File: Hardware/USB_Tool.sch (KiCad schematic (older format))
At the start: 39 parts, among them J1 USB_B_Micro, J2 CONN_ICSP, J3 Extender_I2C_1, J4 Extender_I2C_2, J5 Extender_I2C_3, P1 2V, P2 2V, P3 2V, P4 2V, SW1 SW_2TO1, U1 MRF89XAM8A, U2 NCP114, U3 MCP2210, U4 PIC18F45K40_44, X1 EXTENDER_SPI_1, X2 EXTENDER_IO_1, X3 EXTENDER_IO_2, X4 EXTENDER_IO_3, Y1 DSC6003JI2A

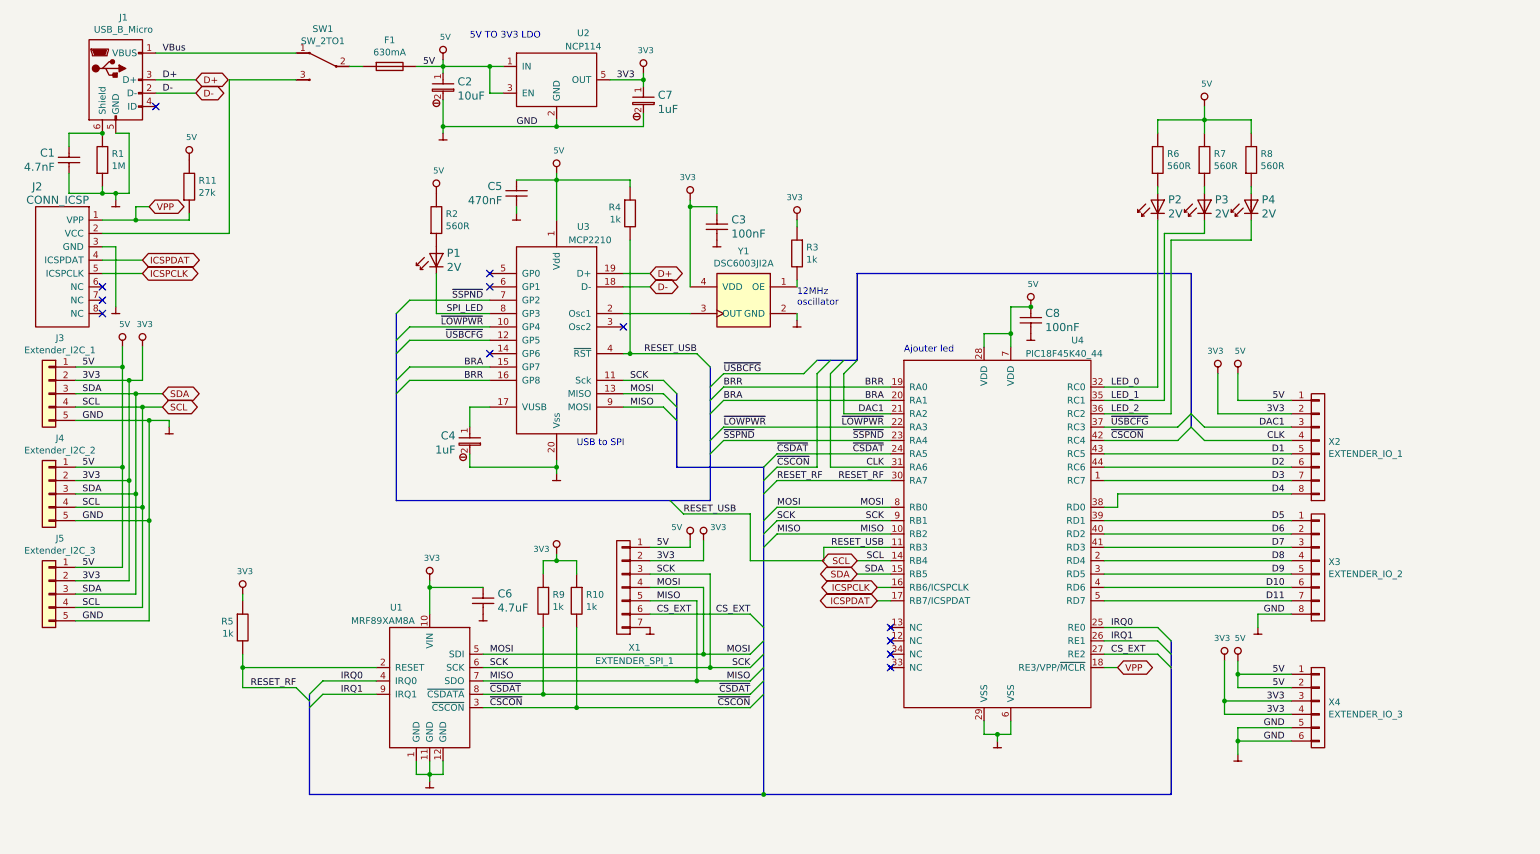
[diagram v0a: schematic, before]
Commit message: tbd
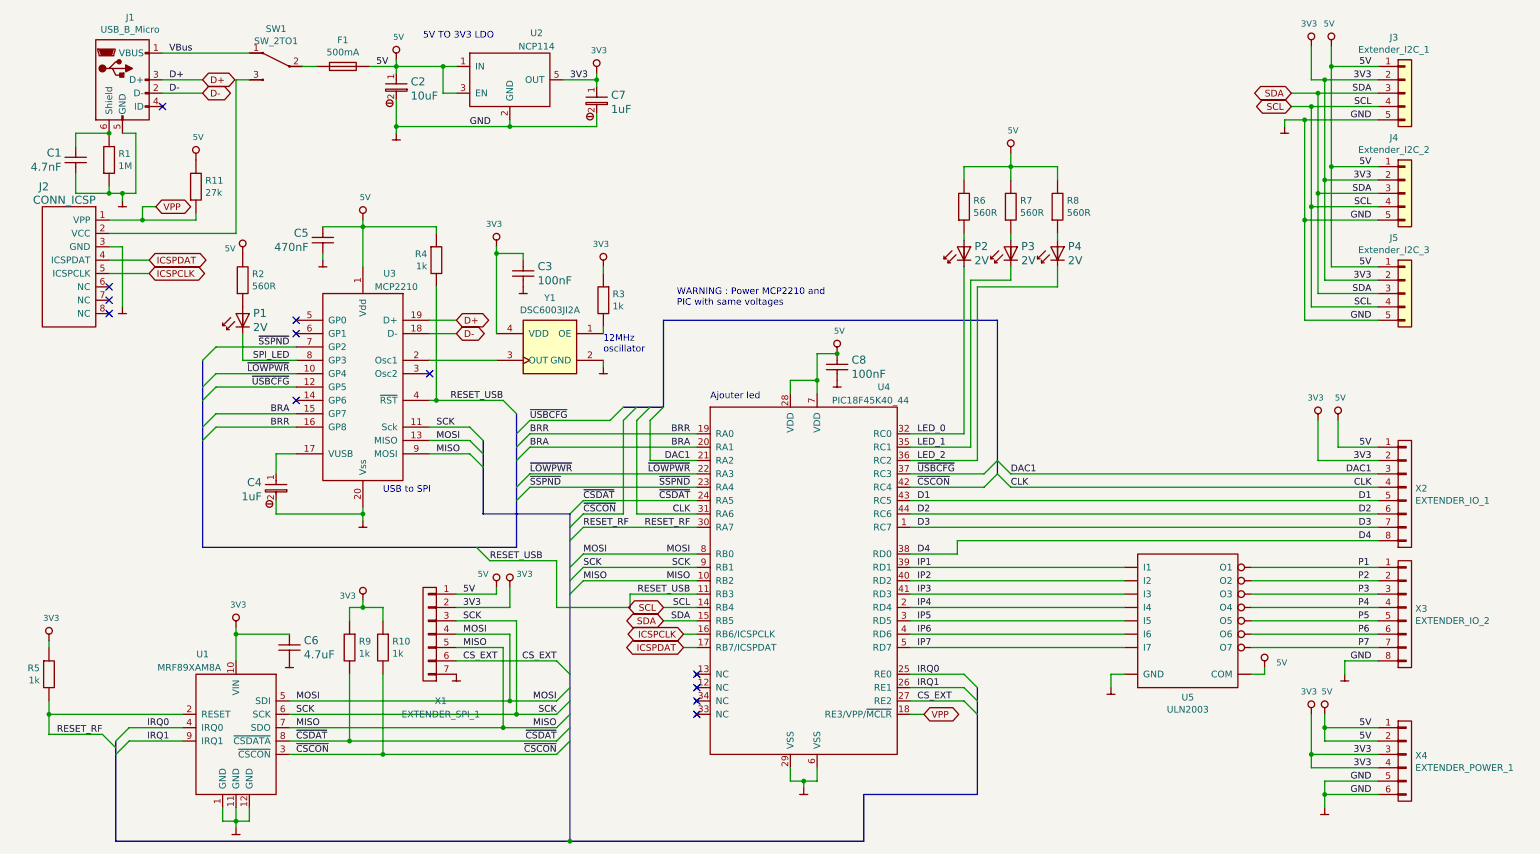
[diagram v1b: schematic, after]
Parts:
- added U5: ULN2003, symbol 0EsseivaN_Lib:ULN200x
- F1: value 630mA -> 500mA
- X4: value EXTENDER_IO_3 -> EXTENDER_POWER_1
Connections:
- net GND: now also U5.8 (GND)
- net VCC: now also U5.9 (COM)
- net D10 renamed IP6
- net IP6: now also U5.6 (I6); no longer X3.6 (P6)
- net D11 renamed IP7
- net IP7: now also U5.7 (I7); no longer X3.7 (P7)
- net D5 renamed IP1
- net IP1: now also U5.1 (I1); no longer X3.1 (P1)
- net D6 renamed IP2
- net IP2: now also U5.2 (I2); no longer X3.2 (P2)
- net D7 renamed IP3
- net IP3: now also U5.3 (I3); no longer X3.3 (P3)
- net D8 renamed IP4
- net IP4: now also U5.4 (I4); no longer X3.4 (P4)
- net D9 renamed IP5
- net IP5: now also U5.5 (I5); no longer X3.5 (P5)
- new net P1: U5.16 (O1), X3.1 (P1)
- new net P2: U5.15 (O2), X3.2 (P2)
- new net P3: U5.14 (O3), X3.3 (P3)
- new net P4: U5.13 (O4), X3.4 (P4)
- new net P5: U5.12 (O5), X3.5 (P5)
- new net P6: U5.11 (O6), X3.6 (P6)
- new net P7: U5.10 (O7), X3.7 (P7)
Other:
- note added: "WARNING : Power MCP2210 and\nPIC with same voltages"
- moved on the sheet: C1, C2, C3, C4, C5, C6, C7, C8, F1, J1, J2, J3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
